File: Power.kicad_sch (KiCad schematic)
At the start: 28 parts

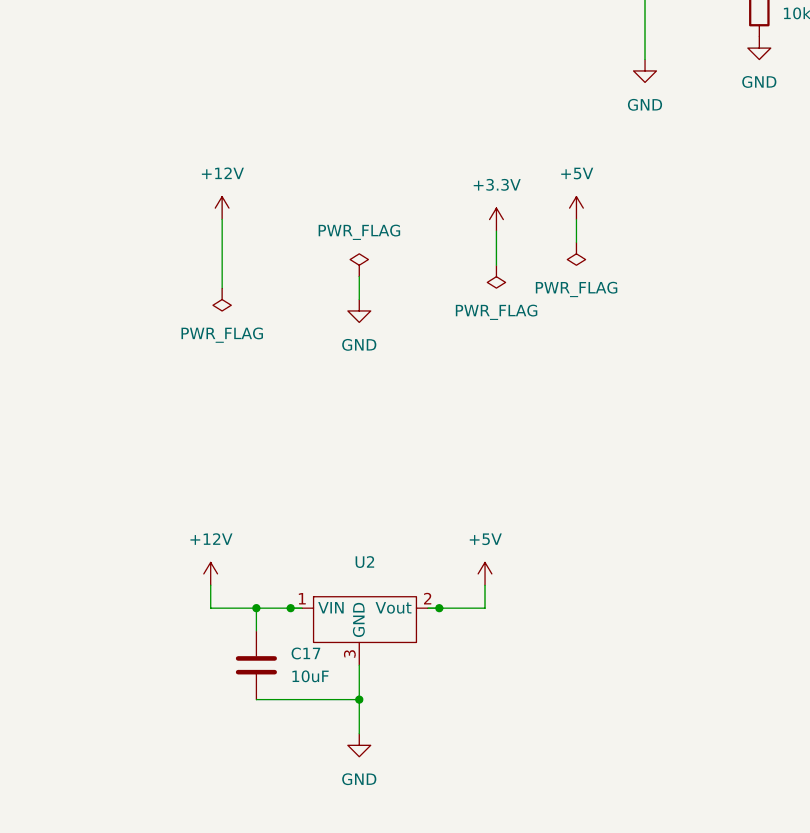
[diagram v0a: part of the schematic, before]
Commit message: Add files via upload
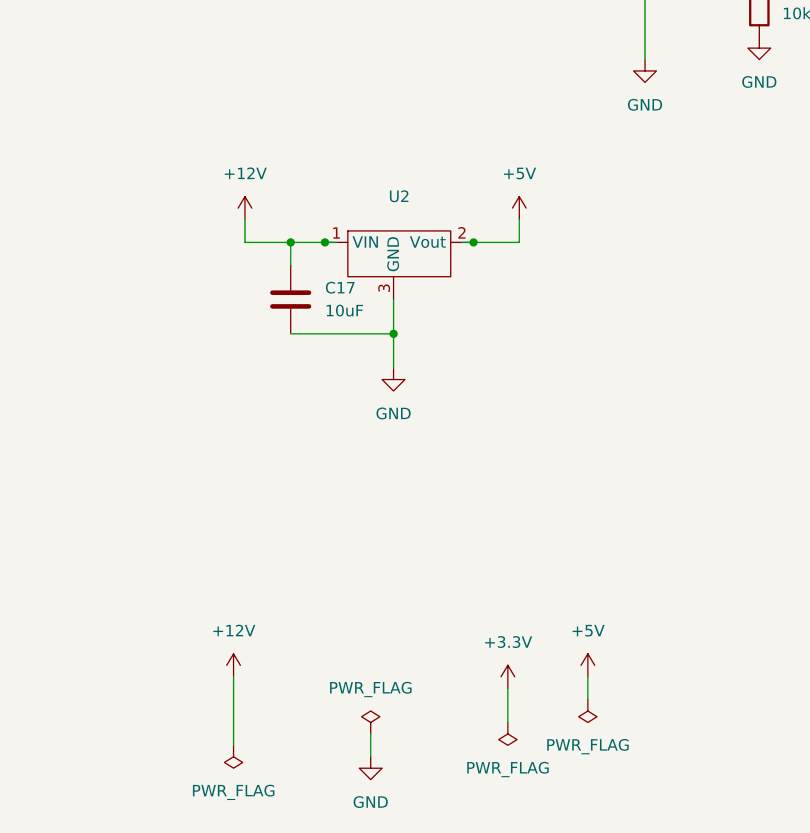
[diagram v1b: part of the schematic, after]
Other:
- moved on the sheet: C17, U2
